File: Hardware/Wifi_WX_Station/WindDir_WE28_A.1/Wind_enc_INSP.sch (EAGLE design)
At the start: 13 parts, among them IC1 EM3242, IC2 TLVB2211, IC3 TC10553.3V

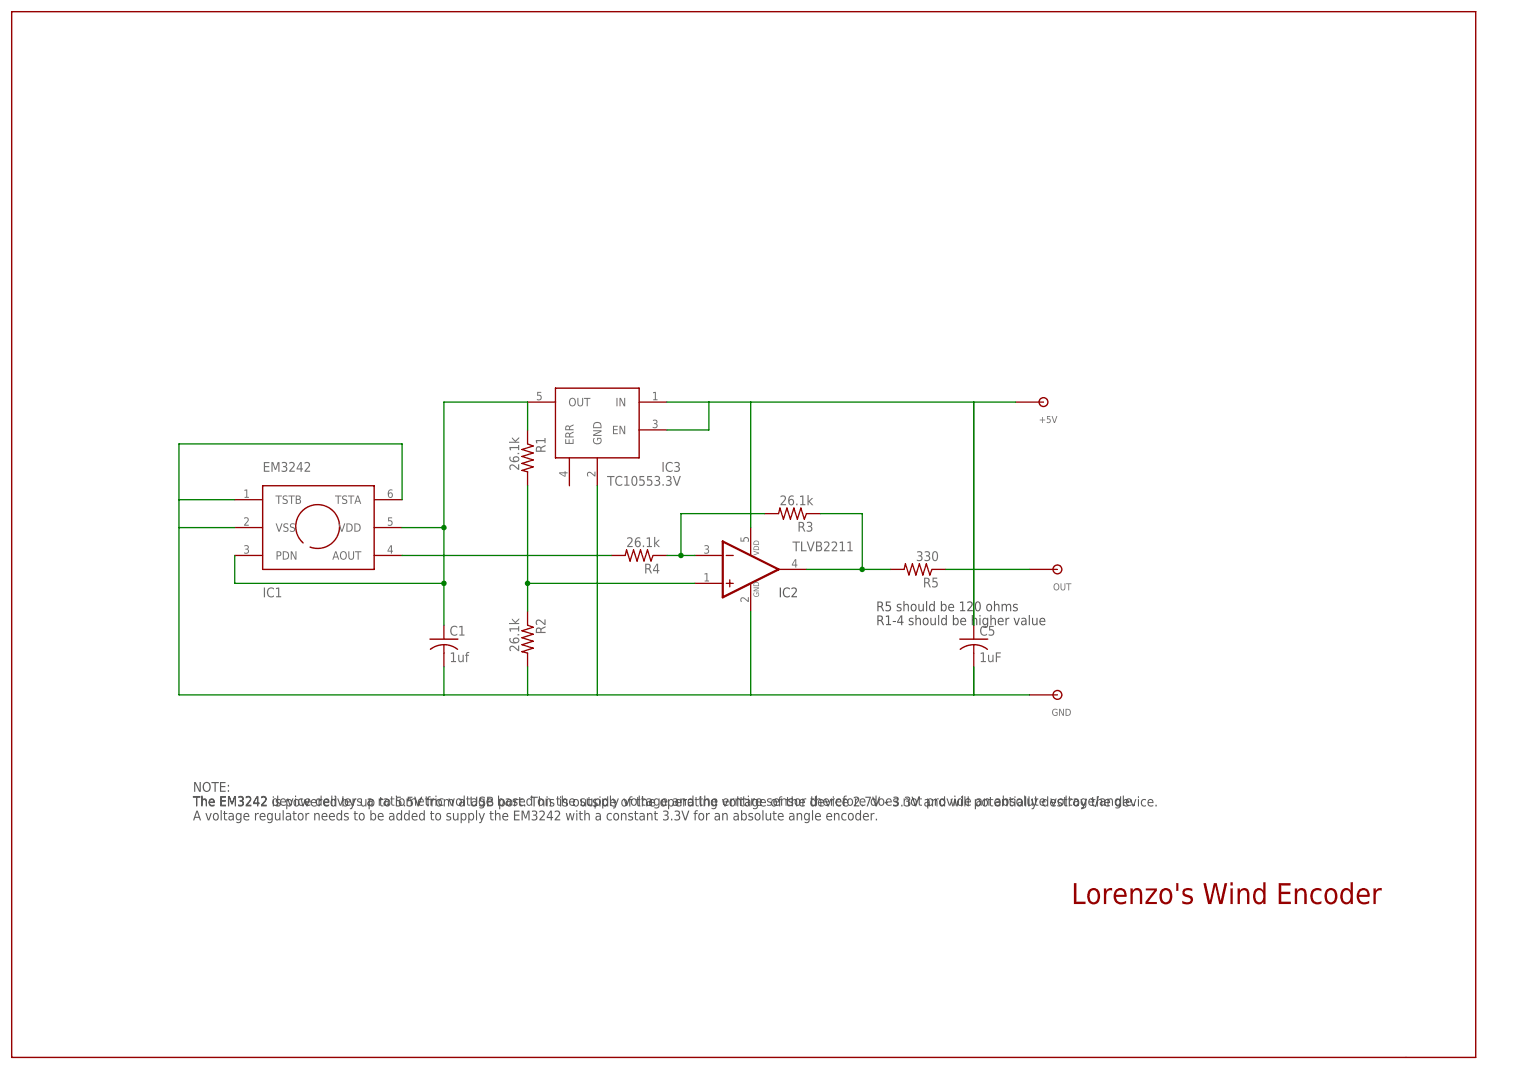
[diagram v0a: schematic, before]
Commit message: backup
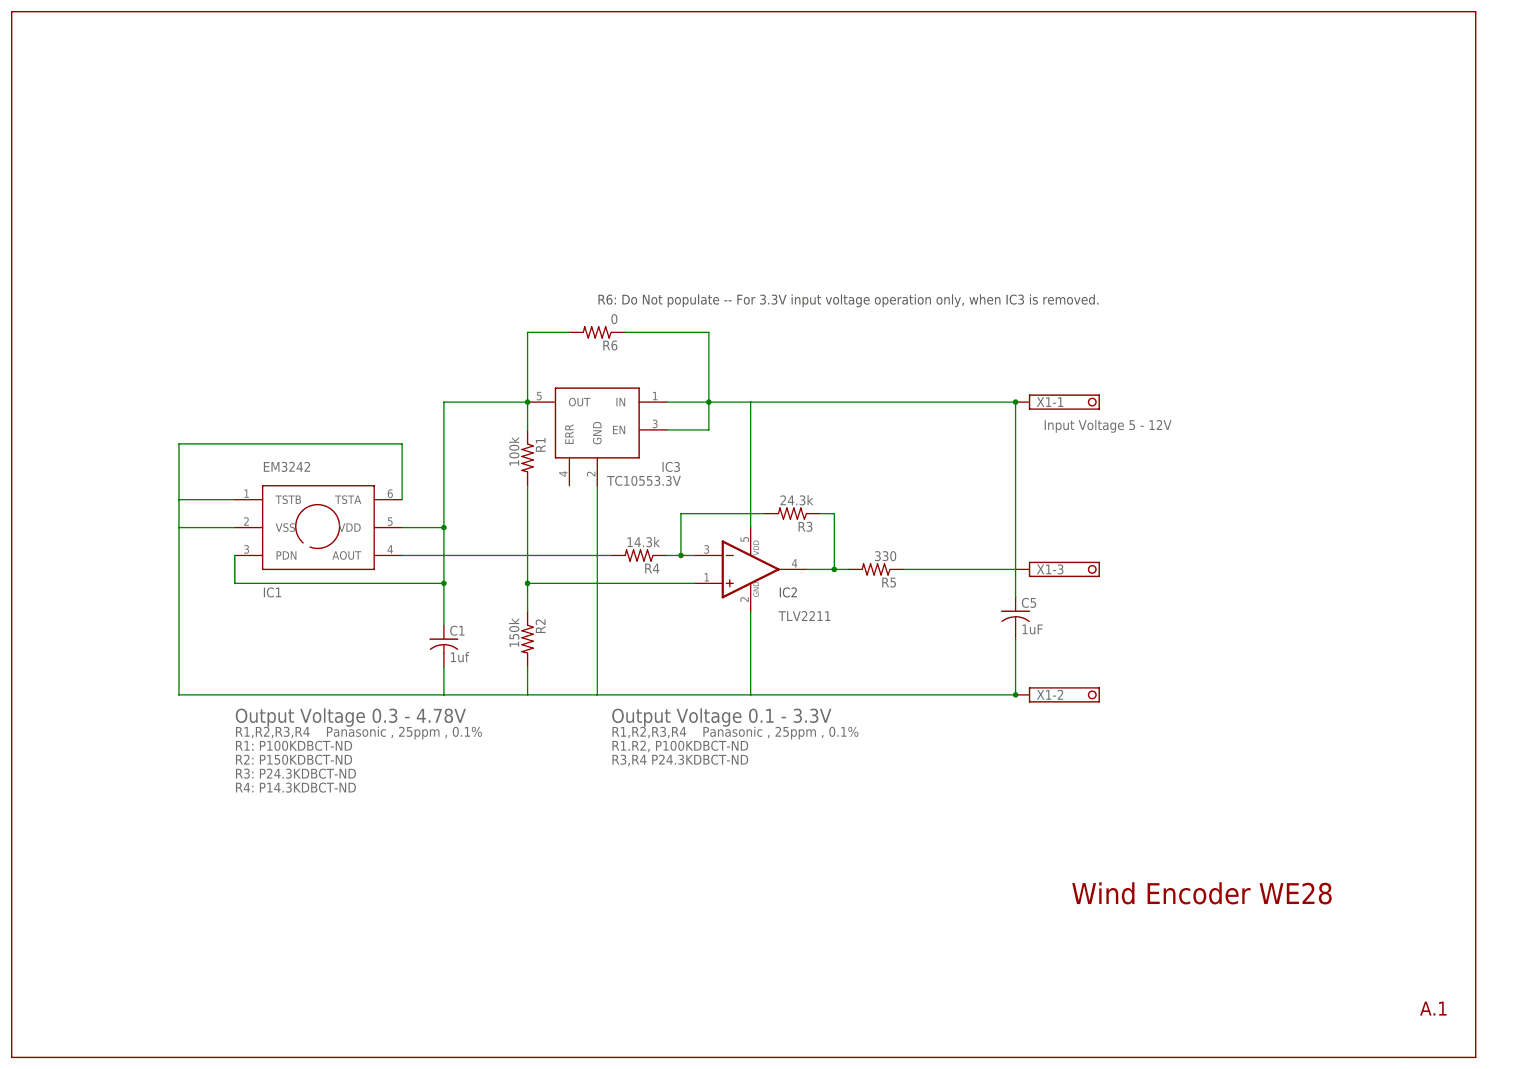
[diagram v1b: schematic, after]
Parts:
- removed +5V, GND, OUT: TPSOL, wifi_WX:TPSOL
- added R6: 0, rcl:R-US_R0603
- added X1: 1751251, con-phoenix-350:1751251
- IC2: value TLVB2211 -> TLV2211
- R1: value 26.1k -> 100k
- R2: value 26.1k -> 150k
- R3: value 26.1k -> 24.3k
- R4: value 26.1k -> 14.3k
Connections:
- net N$1: now also R6.1, X1-1.K; no longer +5V.P$1
- net N$2: now also X1-2.K; no longer GND.P$1
- net N$3: now also X1-3.K; no longer OUT.P$1
- net N$5: now also R6.2
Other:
- note added: "A.1"
- note added: "Input Voltage 5 - 12V"
- note added: "Output Voltage 0.1 - 3.3V"
- note added: "Output Voltage 0.3 - 4.78V"
- note added: "R1,R2,R3,R4 Panasonic , 25ppm , 0.1%"
- note added: "R1.R2, P100KDBCT-ND"
- note added: "R1: P100KDBCT-ND"
- note added: "R2: P150KDBCT-ND"
- note added: "R3,R4 P24.3KDBCT-ND"
- note added: "R3: P24.3KDBCT-ND"
- note added: "R4: P14.3KDBCT-ND"
- note added: "R6: Do Not populate -- For 3.3V input voltage operation only, when IC3 is removed."
- note added: "Wind Encoder WE28"
- note removed: "Lorenzo's Wind Encoder"
- note removed: "NOTE: The EM3242 is powered by up to 5.5V from a USB port. This is outside of the operating voltage of the device 2.7V - 3.3V and will potentially destroy the device."
- note removed: "R1-4 should be higher value"
- note removed: "R5 should be 120 ohms"
- note removed: "The EM3242 device delivers a ratiometric voltage based on the supply voltage and the erntire sensor therefore does not provide an absolute voltage/angle. A voltage regulator needs to be added to supply the EM3242 with a constant 3.3V for an absolute angle encoder."
- moved on the sheet: C5, R5
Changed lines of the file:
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@@
 <?xml version="1.0" encoding="utf-8"?>
 <!DOCTYPE eagle SYSTEM "eagle.dtd">
-<eagle version="6.3">
+<eagle version="6.5.0">
 <drawing>
 <settings>
@@
 </classes>
 <parts>
-<part name="R4" library="rcl" deviceset="R-US_" device="R0603" value="26.1k"/>
+<part name="R4" library="rcl" deviceset="R-US_" device="R0603" value="14.3k"/>
 <part name="C5" library="rcl" deviceset="C-US" device="C0805K" value="1uF"/>
 <part name="C1" library="rcl" deviceset="C-US" device="C0805K" value="1uf"/>
-<part name="OUT" library="wifi_WX" deviceset="TP" device="SOL"/>
-<part name="+5V" library="wifi_WX" deviceset="TP" device="SOL"/>
-<part name="GND" library="wifi_WX" deviceset="TP" device="SOL"/>
-<part name="R1" library="rcl" deviceset="R-US_" device="R0603" value="26.1k"/>
-<part name="R2" library="rcl" deviceset="R-US_" device="R0603" value="26.1k"/>
+<part name="R1" library="rcl" deviceset="R-US_" device="R0603" value="100k"/>
+<part name="R2" library="rcl" deviceset="R-US_" device="R0603" value="150k"/>
 <part name="U$1" library="1AA_Stofer" deviceset="8.5X11" device=""/>
 <part name="IC1" library="1AA_Stofer" deviceset="EM3242" device=""/>
-<part name="IC2" library="1AA_Stofer" deviceset="TLVB2211" device=""/>
-<part name="R3" library="rcl" deviceset="R-US_" device="R0603" value="26.1k"/>
+<part name="IC2" library="1AA_Stofer" deviceset="TLVB2211" device="" value="TLV2211"/>
+<part name="R3" library="rcl" deviceset="R-US_" device="R0603" value="24.3k"/>
 <part name="R5" library="rcl" deviceset="R-US_" device="R0603" value="330"/>
 <part name="IC3" library="1AA_Stofer" deviceset="TC10553.3V" device=""/>
+<part name="X1" library="con-phoenix-350" deviceset="1751251" device=""/>
+<part name="R6" library="rcl" deviceset="R-US_" device="R0603" value="0"/>
 </parts>
 <sheets>
 <sheet>
 <plain>
-<text x="119.38" y="-12.7" size="3.81" layer="94" ratio="20">Lorenzo's Wind Encoder</text>
-<text x="-40.64" y="5.08" size="1.778" layer="97">NOTE:
-The EM3242 is powered by up to 5.5V from a USB port. This is outside of the operating voltage of the device 2.7V - 3.3V and will potentially destroy the device.
-</text>
-<text x="-40.64" y="2.54" size="1.778" layer="97">The EM3242 device delivers a ratiometric voltage based on the supply voltage and the erntire sensor therefore does not provide an absolute voltage/angle.
-A voltage regulator needs to be added to supply the EM3242 with a constant 3.3V for an absolute angle encoder. </text>
-<wire x1="101.6" y1="38.1" x2="101.6" y2="78.74" width="0.1524" layer="97"/>
-<wire x1="101.6" y1="30.48" x2="101.6" y2="25.4" width="0.1524" layer="97"/>
-<text x="83.82" y="40.64" size="1.778" layer="97">R5 should be 120 ohms</text>
-<text x="83.82" y="38.1" size="1.778" layer="97">R1-4 should be higher value </text>
+<text x="119.38" y="-12.7" size="3.81" layer="94" ratio="20">Wind Encoder WE28</text>
 <text x="66.04" y="43.18" size="1.778" layer="97">IC2</text>
+<text x="33.02" y="96.52" size="1.778" layer="97">R6: Do Not populate -- For 3.3V input voltage operation only, when IC3 is removed.</text>
+<text x="182.88" y="-33.02" size="2.54" layer="94">A.1</text>
+<text x="-33.02" y="17.78" size="1.778" layer="96">R1,R2,R3,R4    Panasonic , 25ppm , 0.1% </text>
+<text x="-33.02" y="12.7" size="1.778" layer="96">R2: P150KDBCT-ND</text>
+<text x="-33.02" y="15.24" size="1.778" layer="96">R1: P100KDBCT-ND</text>
+<text x="-33.02" y="10.16" size="1.778" layer="96">R3: P24.3KDBCT-ND</text>
+<text x="-33.02" y="7.62" size="1.778" layer="96">R4: P14.3KDBCT-ND</text>
+<text x="-33.02" y="20.32" size="2.54" layer="96">Output Voltage 0.3 - 4.78V</text>
+<text x="114.3" y="73.66" size="1.778" layer="96">Input Voltage 5 - 12V</text>
+<text x="35.56" y="20.32" size="2.54" layer="96">Output Voltage 0.1 - 3.3V</text>
+<text x="35.56" y="17.78" size="1.778" layer="96">R1,R2,R3,R4    Panasonic , 25ppm , 0.1%</text>
+<text x="35.56" y="15.24" size="1.778" layer="96">R1.R2, P100KDBCT-ND</text>
+<text x="35.56" y="12.7" size="1.778" layer="96">R3,R4 P24.3KDBCT-ND</text>
 </plain>
 <instances>
 <instance part="R4" gate="G$1" x="40.64" y="50.8" rot="R180"/>
-<instance part="C5" gate="G$1" x="101.6" y="35.56"/>
+<instance part="C5" gate="G$1" x="109.22" y="40.64"/>
 <instance part="C1" gate="G$1" x="5.08" y="35.56"/>
-<instance part="OUT" gate="G$1" x="116.84" y="48.26" rot="R180"/>
-<instance part="+5V" gate="G$1" x="114.3" y="78.74" rot="R180"/>
-<instance part="GND" gate="G$1" x="116.84" y="25.4" rot="R180"/>
 <instance part="R1" gate="G$1" x="20.32" y="68.58" rot="R270"/>
 <instance part="R2" gate="G$1" x="20.32" y="35.56" rot="R270"/>
@@
 <instance part="IC1" gate="G$1" x="-25.4" y="48.26"/>
 <instance part="IC2" gate="G$1" x="60.96" y="48.26" smashed="yes" rot="MR180">
-<attribute name="VALUE" x="68.58" y="53.34" size="1.778" layer="96" rot="MR180"/>
+<attribute name="VALUE" x="66.04" y="40.64" size="1.778" layer="96" rot="MR180"/>
 </instance>
 <instance part="IC2" gate="G$2" x="63.5" y="48.26" smashed="yes"/>
 <instance part="R3" gate="G$1" x="68.58" y="58.42" rot="R180"/>
-<instance part="R5" gate="G$1" x="91.44" y="48.26" rot="R180"/>
+<instance part="R5" gate="G$1" x="83.82" y="48.26" rot="R180"/>
 <instance part="IC3" gate="G$1" x="33.02" y="73.66" rot="MR0"/>
+<instance part="X1" gate="-1" x="111.76" y="78.74" smashed="yes">
+<attribute name="NAME" x="113.03" y="77.851" size="1.778" layer="95" font="vector"/>
+</instance>
+<instance part="X1" gate="-2" x="111.76" y="25.4" smashed="yes">
+<attribute name="NAME" x="113.03" y="24.511" size="1.778" layer="95" font="vector"/>
+</instance>
+<instance part="X1" gate="-3" x="111.76" y="48.26" smashed="yes">
+<attribute name="NAME" x="113.03" y="47.371" size="1.778" layer="95" font="vector"/>
+</instance>
+<instance part="R6" gate="G$1" x="33.02" y="91.44" rot="R180"/>
 </instances>
 <busses>
@@
 <wire x1="5.08" y1="25.4" x2="5.08" y2="30.48" width="0.1524" layer="91"/>
 <pinref part="C1" gate="G$1" pin="2"/>
-<pinref part="GND" gate="G$1" pin="P$1"/>
-<wire x1="60.96" y1="25.4" x2="101.6" y2="25.4" width="0.1524" layer="91"/>
+<wire x1="60.96" y1="25.4" x2="109.22" y2="25.4" width="0.1524" layer="91"/>
 <pinref part="IC2" gate="G$2" pin="VDD_GND"/>
-<wire x1="101.6" y1="25.4" x2="111.76" y2="25.4" width="0.1524" layer="91"/>
 <wire x1="60.96" y1="25.4" x2="60.96" y2="40.64" width="0.1524" layer="91"/>
 <wire x1="60.96" y1="25.4" x2="33.02" y2="25.4" width="0.1524" layer="91"/>
@@
 <wire x1="33.02" y1="63.5" x2="33.02" y2="25.4" width="0.1524" layer="91"/>
 <pinref part="C5" gate="G$1" pin="2"/>
-<wire x1="101.6" y1="30.48" x2="101.6" y2="25.4" width="0.1524" layer="91"/>
-</segment>
-</net>
-<net name="N$3" class="0">
-<segment>
-<pinref part="OUT" gate="G$1" pin="P$1"/>
-<wire x1="96.52" y1="48.26" x2="111.76" y2="48.26" width="0.1524" layer="91"/>
-<pinref part="R5" gate="G$1" pin="1"/>
+<wire x1="109.22" y1="35.56" x2="109.22" y2="25.4" width="0.1524" layer="91"/>
+<pinref part="X1" gate="-2" pin="K"/>
+<junction x="109.22" y="25.4"/>
 </segment>
 </net>
@@
 <junction x="5.08" y="55.88"/>
 <pinref part="IC3" gate="G$1" pin="OUT"/>
+<pinref part="R6" gate="G$1" pin="2"/>
+<wire x1="27.94" y1="91.44" x2="20.32" y2="91.44" width="0.1524" layer="91"/>
+<wire x1="20.32" y1="91.44" x2="20.32" y2="78.74" width="0.1524" layer="91"/>
+<junction x="20.32" y="78.74"/>
 </segment>
 </net>
@@
 <segment>
 <pinref part="R3" gate="G$1" pin="1"/>
-<wire x1="73.66" y1="58.42" x2="81.28" y2="58.42" width="0.1524" layer="91"/>
-<wire x1="81.28" y1="58.42" x2="81.28" y2="48.26" width="0.1524" layer="91"/>
+<wire x1="73.66" y1="58.42" x2="76.2" y2="58.42" width="0.1524" layer="91"/>
+<wire x1="76.2" y1="58.42" x2="76.2" y2="48.26" width="0.1524" layer="91"/>
 <pinref part="IC2" gate="G$1" pin="OUT"/>
-<wire x1="81.28" y1="48.26" x2="71.12" y2="48.26" width="0.1524" layer="91"/>
+<wire x1="76.2" y1="48.26" x2="71.12" y2="48.26" width="0.1524" layer="91"/>
 <pinref part="R5" gate="G$1" pin="2"/>
-<wire x1="81.28" y1="48.26" x2="86.36" y2="48.26" width="0.1524" layer="91"/>
-<junction x="81.28" y="48.26"/>
+<wire x1="76.2" y1="48.26" x2="78.74" y2="48.26" width="0.1524" layer="91"/>
+<junction x="76.2" y="48.26"/>
 </segment>
 </net>
@@
 <net name="N$1" class="0">
 <segment>
-<pinref part="+5V" gate="G$1" pin="P$1"/>
-<wire x1="60.96" y1="78.74" x2="101.6" y2="78.74" width="0.1524" layer="91"/>
+<wire x1="60.96" y1="78.74" x2="109.22" y2="78.74" width="0.1524" layer="91"/>
 <pinref part="IC2" gate="G$2" pin="VDD"/>
-<wire x1="101.6" y1="78.74" x2="109.22" y2="78.74" width="0.1524" layer="91"/>
 <wire x1="60.96" y1="55.88" x2="60.96" y2="78.74" width="0.1524" layer="91"/>
 <pinref part="IC3" gate="G$1" pin="IN"/>
@@
 <wire x1="53.34" y1="73.66" x2="53.34" y2="78.74" width="0.1524" layer="91"/>
 <pinref part="C5" gate="G$1" pin="1"/>
-<wire x1="101.6" y1="38.1" x2="101.6" y2="78.74" width="0.1524" layer="91"/>
+<wire x1="109.22" y1="43.18" x2="109.22" y2="78.74" width="0.1524" layer="91"/>
+<pinref part="X1" gate="-1" pin="K"/>
+<junction x="109.22" y="78.74"/>
+<pinref part="R6" gate="G$1" pin="1"/>
+<wire x1="38.1" y1="91.44" x2="53.34" y2="91.44" width="0.1524" layer="91"/>
+<wire x1="53.34" y1="91.44" x2="53.34" y2="78.74" width="0.1524" layer="91"/>
+<junction x="53.34" y="78.74"/>
+</segment>
+</net>
+<net name="N$3" class="0">
+<segment>
+<pinref part="R5" gate="G$1" pin="1"/>
+<pinref part="X1" gate="-3" pin="K"/>
+<wire x1="88.9" y1="48.26" x2="109.22" y2="48.26" width="0.1524" layer="91"/>
 </segment>
 </net>
@@
 </schematic>
 </drawing>
-<compatibility>
-<note version="6.3" minversion="6.2.2" severity="warning">
-Since Version 6.2.2 text objects can contain more than one line,
-which will not be processed correctly with this version.
-</note>
-</compatibility>
 </eagle>
